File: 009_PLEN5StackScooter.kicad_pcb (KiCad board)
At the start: 2 copper layers, 80 x 50 mm, 30 parts, among them IC1 NJM2845DL1-33-TE1, IC2 TB6608FNG_O,EL_, IC3 TB6608FNG_O,EL_, J1 S4B-XH-A-1_LF__SN_, J2 S5B-XH-A-1_LF__SN_, J3 S4B-XH-A-1_LF__SN_, J4 S4B-XH-A-1_LF__SN_, Q1 IRLML6402, SW1 SW_OTAX-Toggle

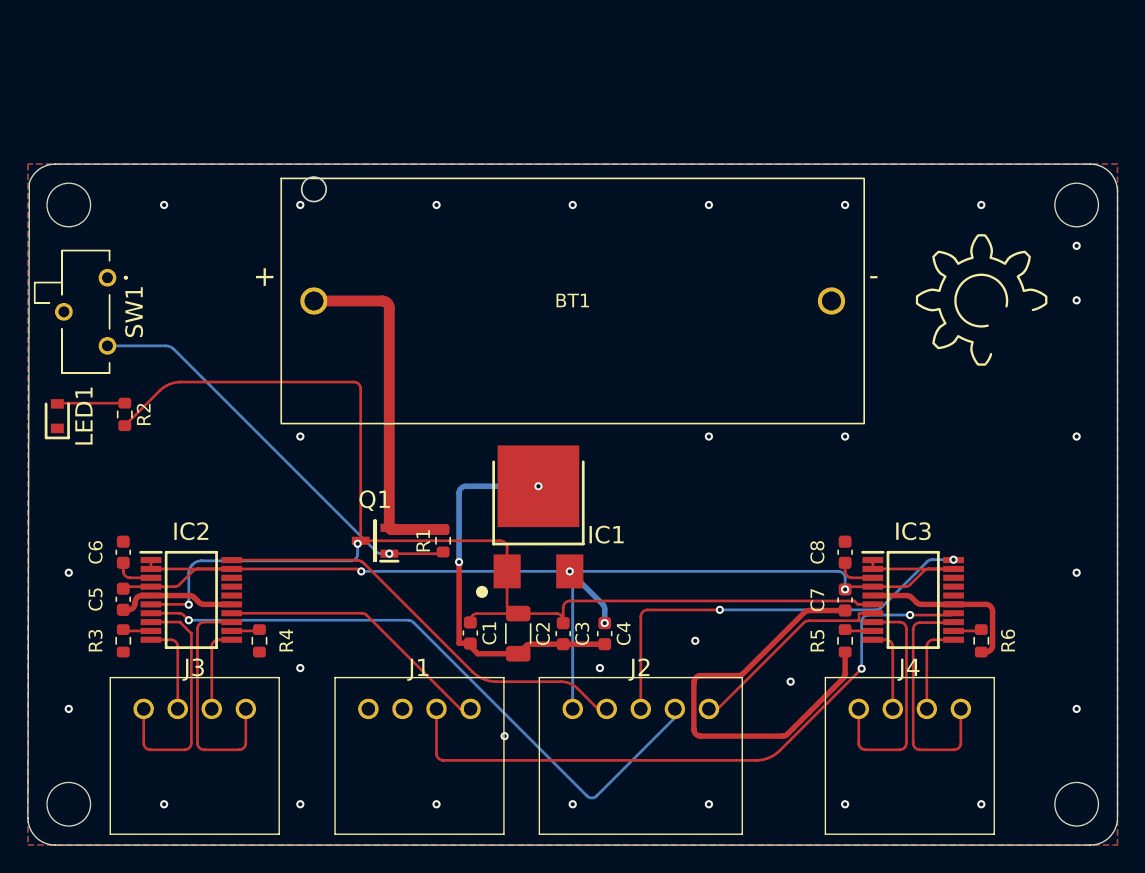
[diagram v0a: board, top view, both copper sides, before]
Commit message: [Add]最終レイアウトに近い基板設計完
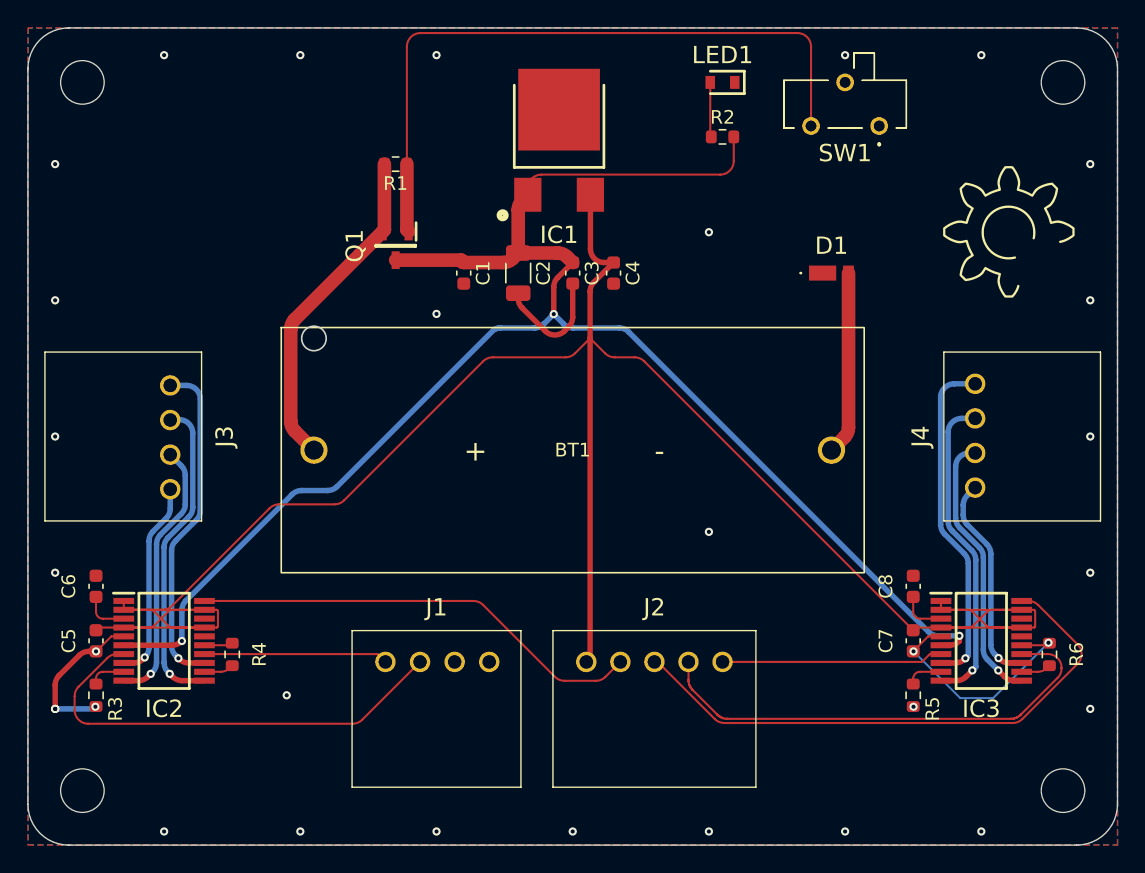
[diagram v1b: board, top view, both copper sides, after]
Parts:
- removed the Ref** at (157.0, 73.0)
- removed the Ref** at (83.0, 117.0)
- removed the Ref** at (83.0, 73.0)
- removed the Ref** at (157.0, 117.0)
- added D1: CUHS20F30,H3F, 01_AddLibrary:CUHS20F30H3F, F.Cu at (139.0, 78.0)
- added Ref**: Val**, 10_KBD_Hole_salicylic:m3_Screw_Hole_EdgeCuts, F.Cu at (156.0, 116.0)
- added Ref**: Val**, 10_KBD_Hole_salicylic:m3_Screw_Hole_EdgeCuts, F.Cu at (84.0, 64.0)
- added Ref**: Val**, 10_KBD_Hole_salicylic:m3_Screw_Hole_EdgeCuts, F.Cu at (156.0, 64.0)
- added Ref**: Val**, 10_KBD_Hole_salicylic:m3_Screw_Hole_EdgeCuts, F.Cu at (84.0, 116.0)
- moved SW1 57.7 mm to (142.5, 67.2), turned to 180 degrees
- moved LED1 54.6 mm to (131.0, 64.0), turned to 180 degrees
- moved R2 48.4 mm to (131.0, 68.0), turned to 0 degrees
- moved R1 27.9 mm to (107.0, 70.0), turned to 180 degrees
- moved IC1 27.7 mm to (119.0, 64.2)
- moved C3 26.5 mm to (120.0, 78.0)
- moved C4 26.5 mm to (123.0, 78.0)
- moved C2 26.5 mm to (116.0, 78.0)
- moved C1 26.4 mm to (112.0, 78.0)
- moved J4 23.8 mm to (149.6, 86.2), turned to -90 degrees
- moved Q1 21.7 mm to (107.0, 76.0), turned to -90 degrees
- moved J3 17.2 mm to (90.5, 93.8), turned to 90 degrees
- moved BT1 11.0 mm to (101.0, 91.0)
- moved R5 6.40 mm to (145.0, 109.0)
- moved C7 5.83 mm to (145.0, 105.0)
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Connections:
- BT1 pad 2: GND -> Net-(BT1--)
- IC2 pad 17: unconnected-(IC2-TQ-Pad17) -> +3.3V
- IC3 pad 17: unconnected-(IC3-TQ-Pad17) -> +3.3V
- J1 pad 2: Reset_2 -> Direction_1
- J2 pad 4: Direction_1 -> Reset_2
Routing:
- net +3.3V: track 91.3 -> 172.4 mm, vias 4 -> 0
- net GND: track 82.3 -> 40.1 mm, vias 31 -> 32
- net +BATT: track 97.4 -> 125.2 mm, vias 2 -> 3
- net Net-(Q1-G): track 30.9 -> 50.2 mm, vias 1 -> 0
- net MotorA2: track 6.30 -> 23.5 mm, vias 0 -> 1
- net MotorB3: track 6.30 -> 23.4 mm, vias 0 -> 1
- net Net-(BT1--): track 0.00 -> 13.5 mm
- net Direction_1: track 47.1 -> 33.8 mm, vias 1 -> 0
- net MotorA4: track 6.80 -> 20.1 mm, vias 0 -> 1
- net MotorB1: track 6.80 -> 19.5 mm, vias 0 -> 1
- net Reset_2: track 47.9 -> 35.3 mm, vias 2 -> 0
- net Clock_2: track 31.5 -> 41.5 mm, vias 2 -> 0
- net MotorB4: track 17.6 -> 24.9 mm, vias 0 -> 1
- net MotorA1: track 17.8 -> 24.7 mm, vias 0 -> 1
- net Reset_1: track 20.4 -> 13.5 mm
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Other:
- board size 80 x 50 mm -> 80 x 60 mm
- board text added: "PLEN5StackScooter_TestBoard v2.0"
- board text removed: "PLEN5StackScooter_TestBoard v1.0"
